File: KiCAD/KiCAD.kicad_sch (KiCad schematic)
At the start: 18 parts, among them J1 RC Channel: Throttle, J2 RC Channel: Steering, J3 RC Channel: Emergency Stop, M1 Motor Controller, M2 Linear Actuator/Servo

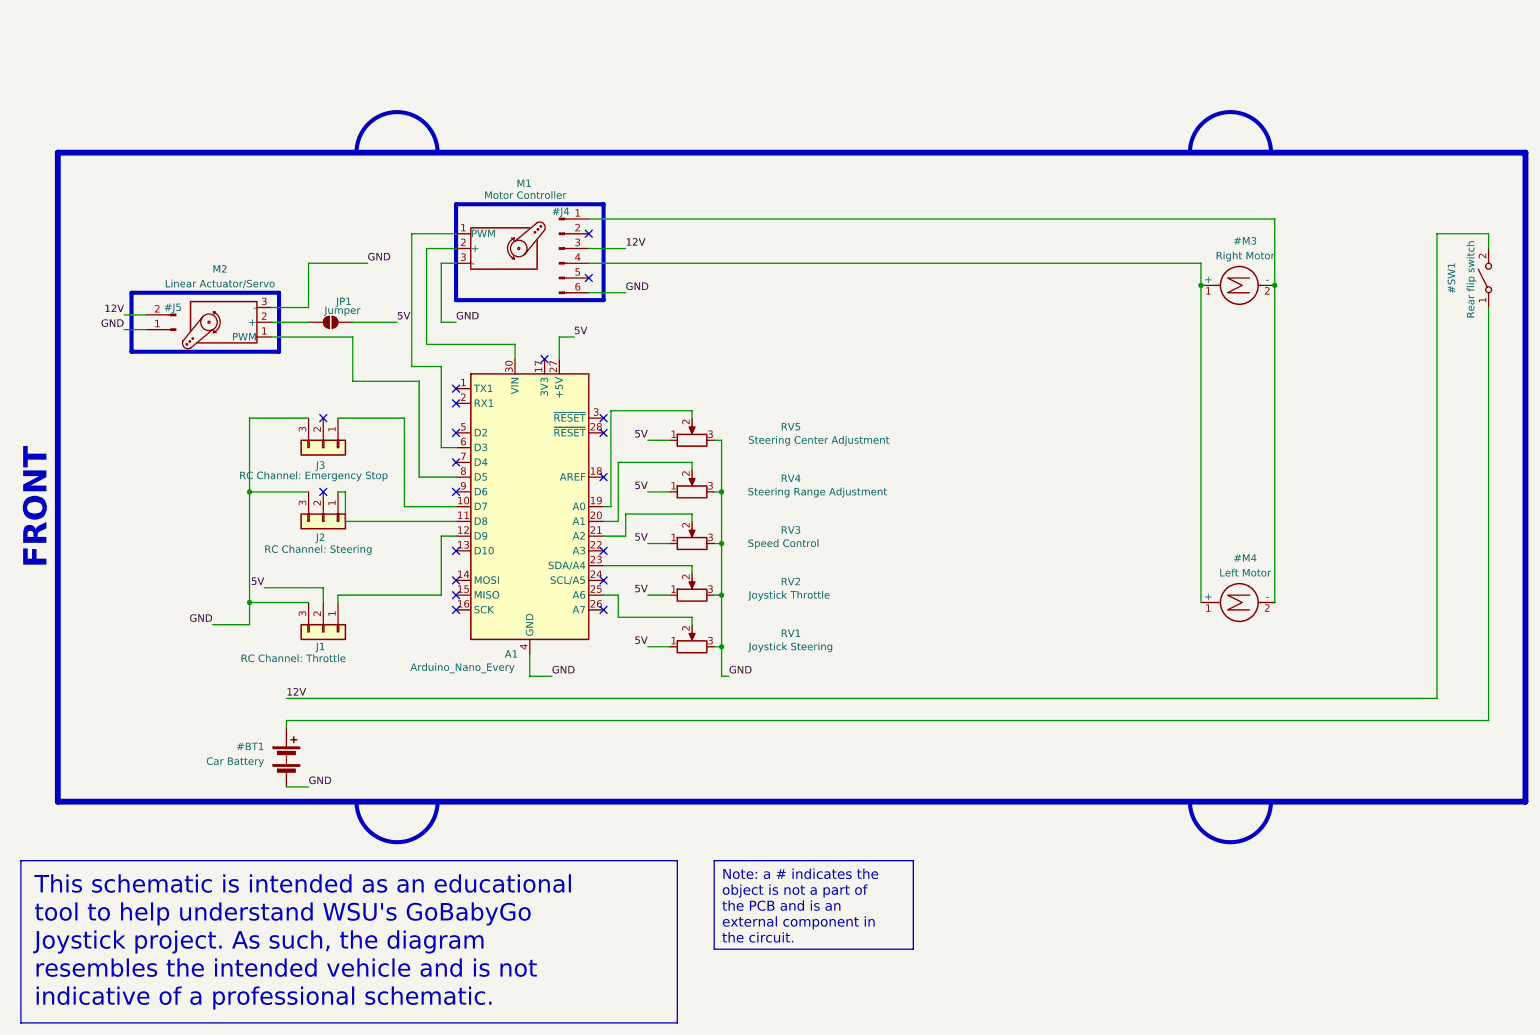
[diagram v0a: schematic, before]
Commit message: update photos and readme
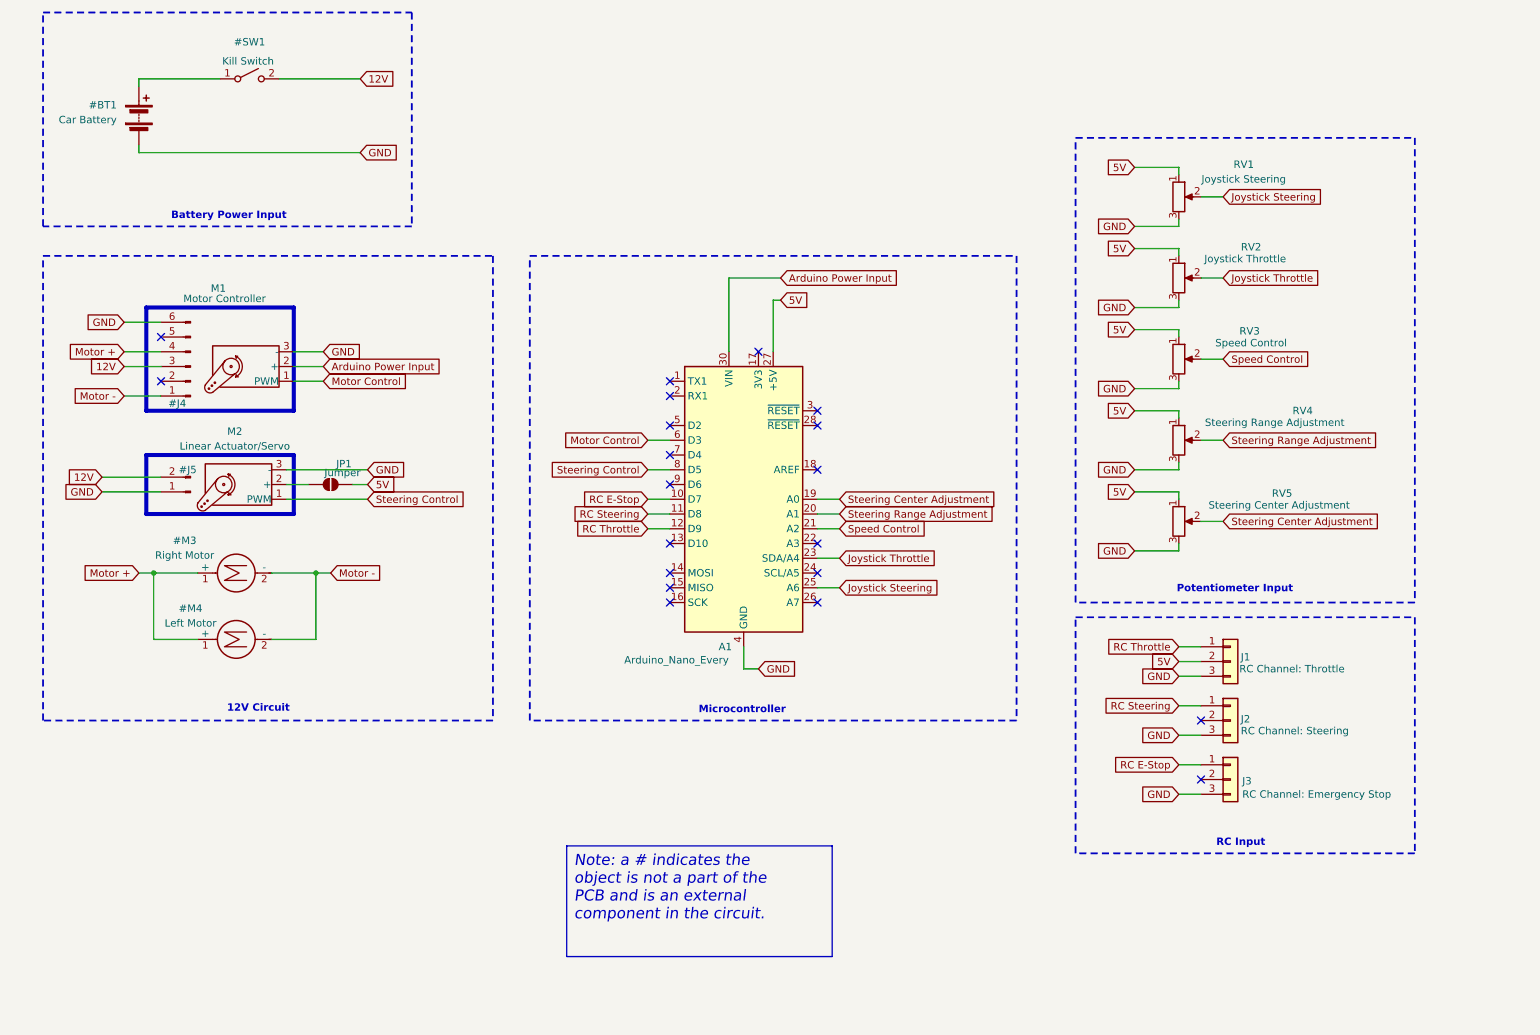
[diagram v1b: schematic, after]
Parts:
- #SW1: value Rear flip switch -> Kill Switch
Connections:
- net Steering Control: now reaches A1.8 (D5), M2.1 (PWM)
- net Steering Range Adjustment: now reaches A1.20 (A1), RV4.2
- net Joystick Steering: now reaches A1.25 (A6), RV1.2
- net Motor Control: now reaches A1.6 (D3), M1.1 (PWM)
- net Arduino Power Input: now reaches A1.30 (VIN), M1.2 (+)
- net RC E-Stop: now reaches A1.10 (D7), J3.1 (Pin_1)
- net RC Steering: now reaches A1.11 (D8), J2.1 (Pin_1)
- net RC Throttle: now reaches A1.12 (D9), J1.1 (Pin_1)
- net Steering Center Adjustment: now reaches A1.19 (A0), RV5.2
- net Speed Control: now reaches A1.21 (A2), RV3.2
- net Joystick Throttle: now reaches A1.23 (SDA/A4), RV2.2
- net Motor +: now reaches #J4.4 (Pin_4), #M3.1 (+), #M4.1 (+)
- net Motor -: now reaches #J4.1 (Pin_1), #M3.2 (-), #M4.2 (-)
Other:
- note added: "12V Circuit"
- note added: "Battery Power Input"
- note added: "Microcontroller"
- note added: "Potentiometer Input"
- note added: "RC Input"
- note removed: "FRONT"
- moved on the sheet: A1, J1, J2, J3, JP1, M1, M2, RV1, RV2, RV3, RV4, RV5
